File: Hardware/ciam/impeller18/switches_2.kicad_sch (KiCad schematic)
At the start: 85 parts, among them J11 430451000, J12 430450600, J13 430450400, J14 430450600, Q23 BSS138, Q24 BSS138, Q25 BSS138, Q26 BSS138, Q27 BSS138, Q28 BSS138, Q29 BSS138, Q30 BSS138, Q31 BSS138, Q32 BSS138, Q33 BSS138, Q34 BSS138, Q35 BSS138, U27 TLP291-4, U28 TLP291-4, U29 B0505MT-1WR4, U30 TLP291, U31 TLP291, U32 TLP291, U33 TLP291, U34 TLP291

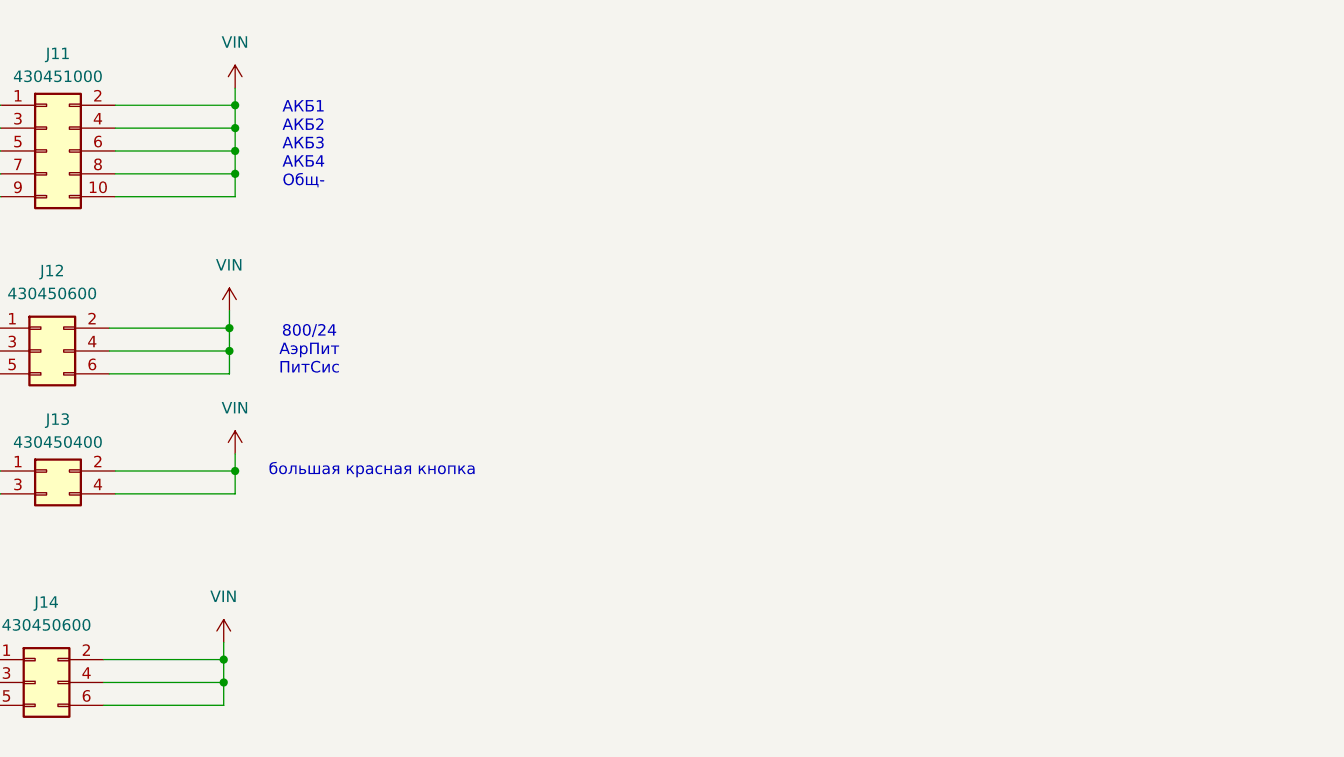
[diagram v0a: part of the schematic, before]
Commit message: bugfixes
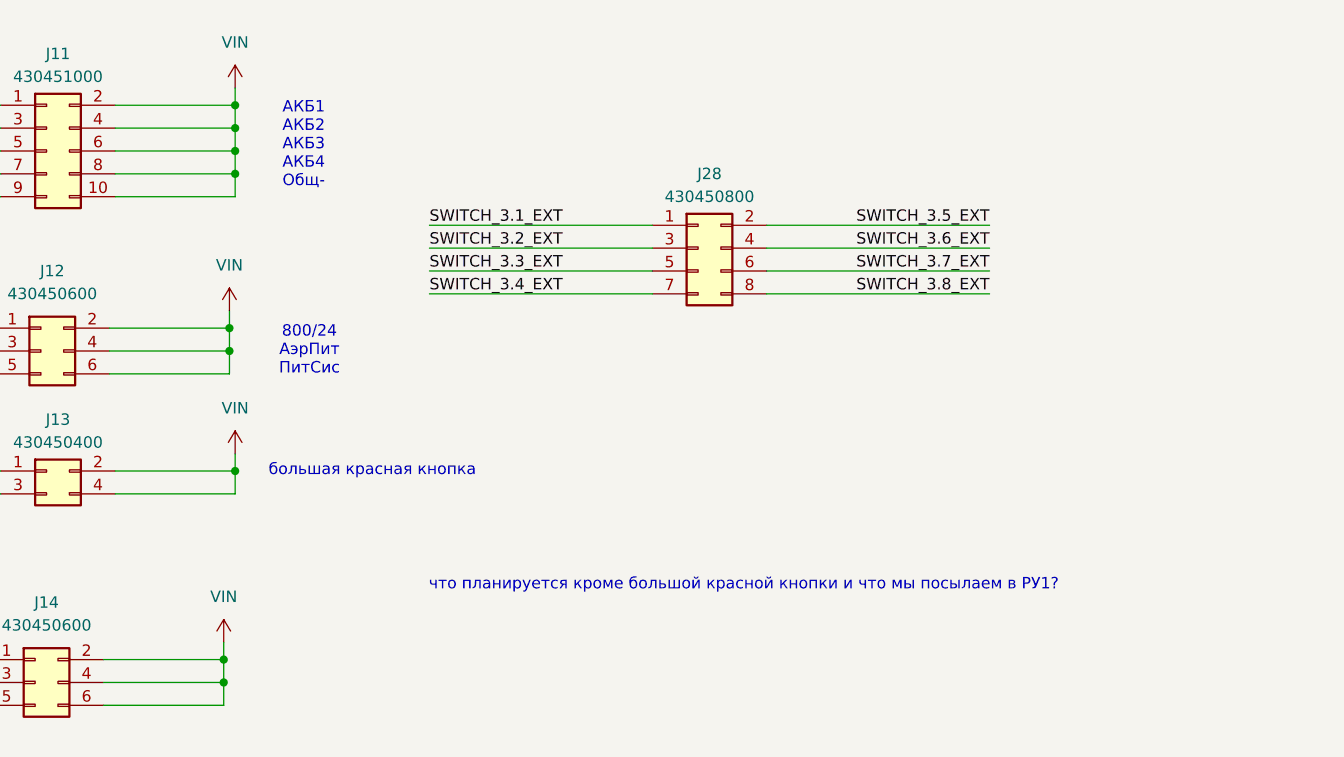
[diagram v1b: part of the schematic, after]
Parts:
- added J28: 430450800, Connector_Molex:Molex_Micro-Fit_3.0_43045-0800_2x04_P3.00mm_Horizontal, symbol Connector_Generic:Conn_02x04_Odd_Even
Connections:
- net SWITCH_3.1_EXT: now also J28.1 (Pin_1)
- net SWITCH_3.2_EXT: now also J28.3 (Pin_3)
- net SWITCH_3.3_EXT: now also J28.5 (Pin_5)
- net SWITCH_3.4_EXT: now also J28.7 (Pin_7)
- net SWITCH_3.5_EXT: now also J28.2 (Pin_2)
- net SWITCH_3.6_EXT: now also J28.4 (Pin_4)
- net SWITCH_3.7_EXT: now also J28.6 (Pin_6)
- net SWITCH_3.8_EXT: now also J28.8 (Pin_8)
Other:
- note added: "что планируется кроме большой красной кнопки и что мы посылаем в РУ1?"
